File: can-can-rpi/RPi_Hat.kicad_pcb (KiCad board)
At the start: 2 copper layers, 65 x 56 mm, 46 parts, among them CON1 BARREL_JACK, J1 RPi_GPIO, P1 CONN_02X02, P2 CONN_01X14, P3 CONN_01X14, P4 CONN_01X02, P5 CONN_01X03, U1 PIC18F25K80, U2 MCP2562-I/P, Y1 16MHz

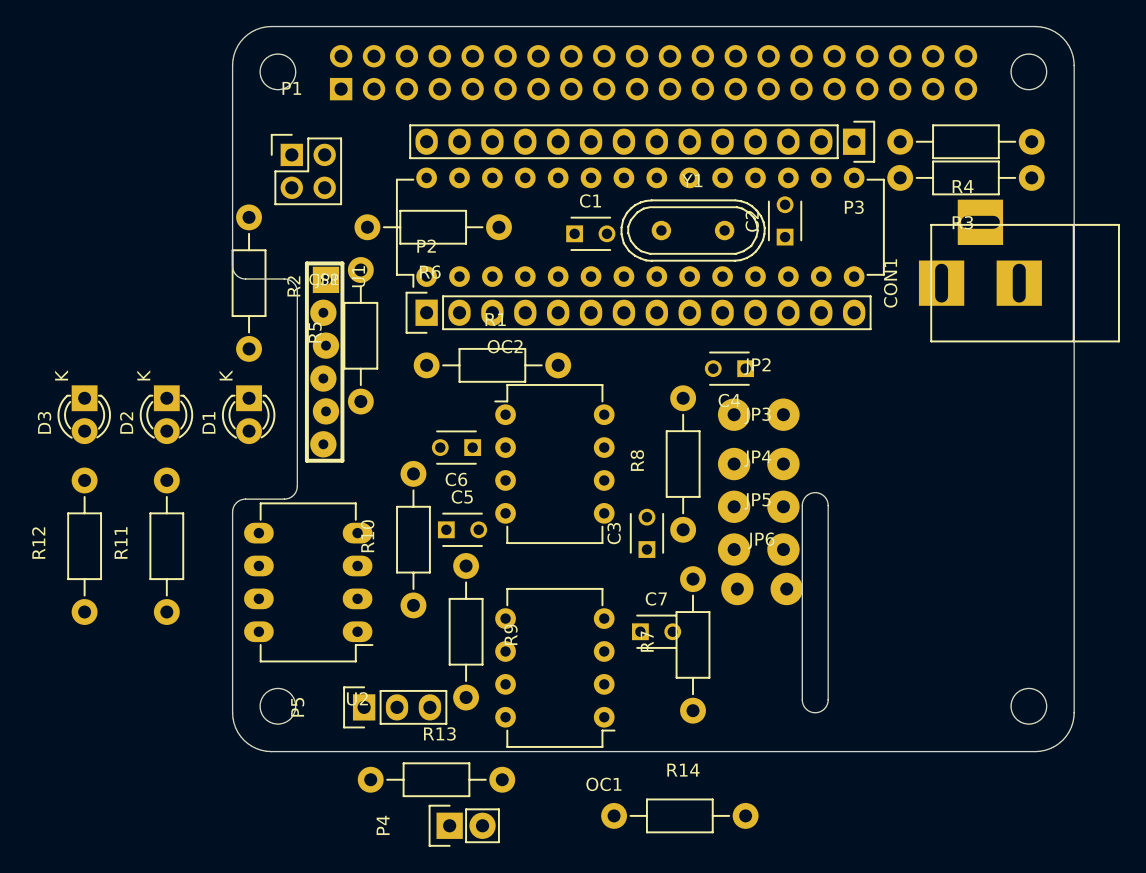
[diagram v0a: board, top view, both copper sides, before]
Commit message: change footprints and layout - wip
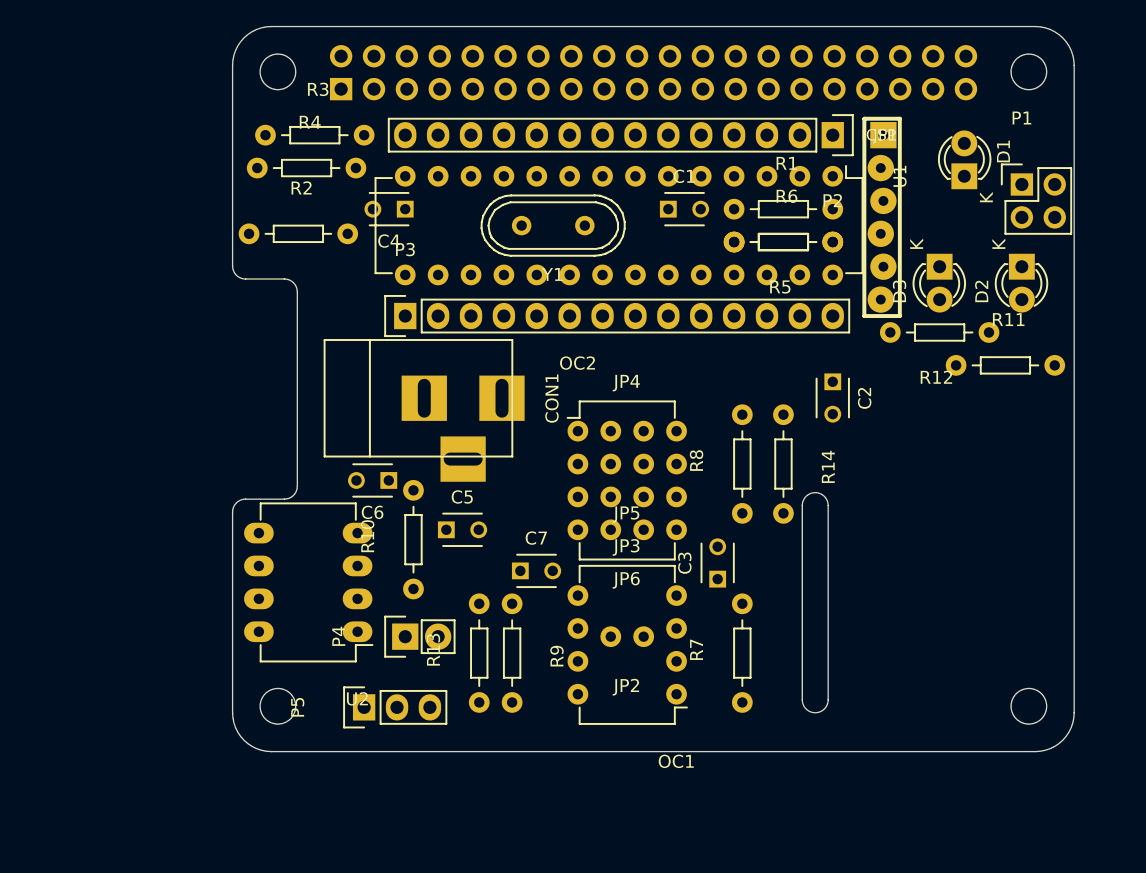
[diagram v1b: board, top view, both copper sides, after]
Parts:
- C3, C4: value 27pF -> 22pF
- JP2, JP3, JP4, JP5, JP6: footprint Wire_Pads:SolderWirePad_2x_1mmDrill -> Wire_Pads:SolderWirePad_2x_0-2.54mmDrill
- R1: value 15k -> 4.7k; footprint Resistors_ThroughHole:Resistor_Horizontal_RM10mm -> Resistors_ThroughHole:Resistor_Horizontal_RM7.5mm
- R10, R11, R12, R13, R14, R2, R3, R4, R7, R8, R9: footprint Resistors_ThroughHole:Resistor_Horizontal_RM10mm -> Resistors_ThroughHole:Resistor_Horizontal_RM7.5mm
- R5, R6: value 470 -> 390; footprint Resistors_ThroughHole:Resistor_Horizontal_RM10mm -> Resistors_ThroughHole:Resistor_Horizontal_RM7.5mm
- moved R12 68.1 mm to (141.0, 95.2), turned to 180 degrees
- moved D2 66.8 mm to (147.3, 90.2)
- moved D3 66.8 mm to (141.0, 90.2)
- moved R11 66.3 mm to (146.1, 97.8), turned to 0 degrees
- moved D1 57.8 mm to (142.9, 83.2), turned to 90 degrees
- moved P1 56.4 mm to (147.3, 83.8)
- moved R4 51.0 mm to (92.1, 82.5), turned to 0 degrees
- moved R3 50.4 mm to (92.7, 80.0), turned to 0 degrees
- moved CON1 47.2 mm to (101.0, 100.3), turned to 0 degrees
- moved JP1 44.5 mm to (136.5, 80.0)
- moved P3 37.2 mm to (99.7, 94.0), turned to 0 degrees
- moved P2 34.2 mm to (132.7, 80.0), turned to 180 degrees
- moved R5 33.4 mm to (128.9, 88.3), turned to 180 degrees
- moved U1 32.3 mm to (132.7, 83.2), turned to 270 degrees
- moved C4 29.0 mm to (99.7, 85.7)
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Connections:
- D1 pad 1: /RPi_GPIO/RA2 -> /RPi_GPIO/RA0
- D3 pad 1: /RPi_GPIO/RA0 -> /RPi_GPIO/RA2
- OC1 pad 2: VCC -> Net-(OC1-Pad2)
- OC1 pad 3: Net-(OC1-Pad3) -> /RPi_GPIO/CANTX
- OC2 pad 2: +5V -> Net-(OC2-Pad2)
- OC2 pad 3: Net-(OC2-Pad3) -> /RPi_GPIO/_CANRX
- OC2 pad 6: /RPi_GPIO/CANTX -> /RPi_GPIO/CANRX
- R10 pad 1: /RPi_GPIO/_CANRX -> Net-(OC2-Pad2)
- R10 pad 2: Net-(OC2-Pad3) -> +5V
- R12 pad 2: Net-(D1-Pad2) -> Net-(D3-Pad2)
- R14 pad 2: /RPi_GPIO/CANTX -> /RPi_GPIO/CANRX
- R2 pad 2: Net-(D3-Pad2) -> Net-(D1-Pad2)
- R7 pad 1: Net-(OC1-Pad3) -> Net-(OC1-Pad2)
- R7 pad 2: /RPi_GPIO/CANTX -> VCC
- R8 pad 1: /RPi_GPIO/CANTX -> /RPi_GPIO/CANRX
